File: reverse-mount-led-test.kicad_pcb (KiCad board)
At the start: 2 copper layers, 12.7 x 12.7 mm, 9 parts, among them J1 Conn_01x02

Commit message: setup design rules
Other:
- net class Default: clearance 0.2 -> 0.254; trace_width 0.25 -> 0.254; via_dia 0.8 -> 0.6858; via_drill 0.4 -> 0.3302
- rule pad_to_mask_clearance: 0.051 -> 0.0508
- rule solder_mask_min_width: 0.25 -> 0.254
- rule trace_clearance: 0.2 -> 0.254
- rule trace_min: 0.2 -> 0.1524
- rule via_min_drill: 0.3 -> 0.3302
- rule via_min_size: 0.4 -> 0.6858
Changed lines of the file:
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@@
   )
   (setup
-    (last_trace_width 0.25)
-    (trace_clearance 0.2)
+    (last_trace_width 0.254)
+    (trace_clearance 0.254)
     (zone_clearance 0.508)
     (zone_45_only no)
-    (trace_min 0.2)
+    (trace_min 0.1524)
     (segment_width 0.2)
     (edge_width 0.15)
-    (via_size 0.8)
-    (via_drill 0.4)
-    (via_min_size 0.4)
-    (via_min_drill 0.3)
+    (via_size 0.6858)
+    (via_drill 0.3302)
+    (via_min_size 0.6858)
+    (via_min_drill 0.3302)
     (uvia_size 0.3)
     (uvia_drill 0.1)
@@
     (pad_size 1.524 1.524)
     (pad_drill 0.762)
-    (pad_to_mask_clearance 0.051)
-    (solder_mask_min_width 0.25)
+    (pad_to_mask_clearance 0.0508)
+    (solder_mask_min_width 0.254)
     (aux_axis_origin 0 0)
     (visible_elements FFFFFF7F)
@@
   (net 6 "Net-(D4-Pad1)")
   (net_class Default "This is the default net class."
-    (clearance 0.2)
-    (trace_width 0.25)
-    (via_dia 0.8)
-    (via_drill 0.4)
+    (clearance 0.254)
+    (trace_width 0.254)
+    (via_dia 0.6858)
+    (via_drill 0.3302)
     (uvia_dia 0.3)
     (uvia_drill 0.1)

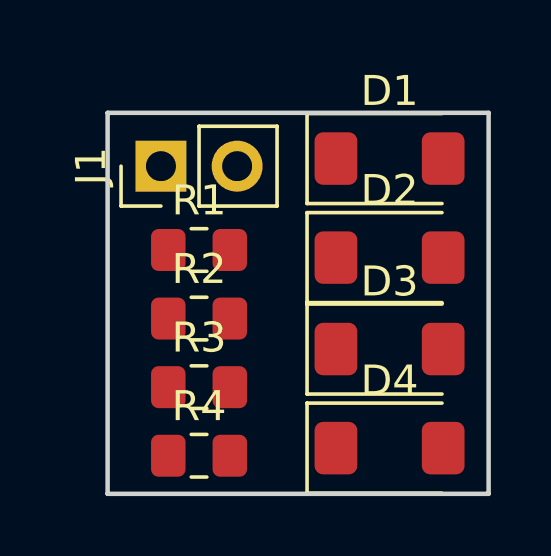
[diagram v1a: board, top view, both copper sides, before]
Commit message: layout done
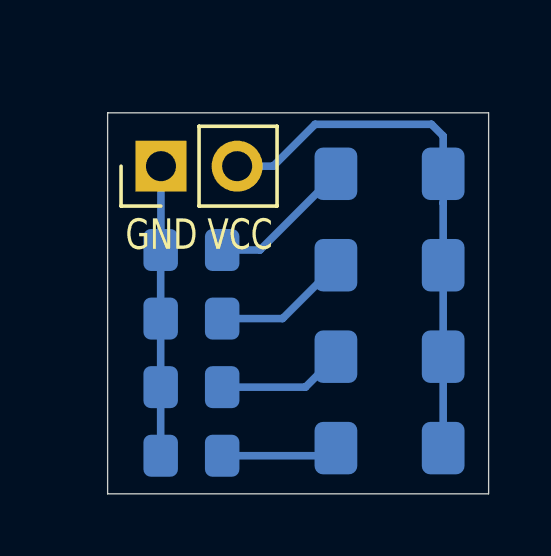
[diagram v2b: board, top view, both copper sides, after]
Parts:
- D1, D2, D3, D4, R1, R2, R3, R4: moved to B.Cu
- moved D1 0.51 mm to (161.8, 103.6)
- moved R1 0.25 mm to (155.2, 106.2)
- moved R2 0.25 mm to (155.2, 108.5)
- moved R3 0.25 mm to (155.2, 110.7)
- moved R4 0.25 mm to (155.2, 113.0)
- moved D2 0.25 mm to (161.8, 106.7)
- moved D3 0.25 mm to (161.8, 109.7)
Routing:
- net VCC: track 0.00 -> 18.0 mm
- net GND: track 0.00 -> 9.67 mm
- net Net-(D1-Pad1): track 0.00 -> 4.86 mm
- net Net-(D2-Pad1): track 0.00 -> 4.53 mm
- net Net-(D3-Pad1): track 0.00 -> 4.21 mm
- net Net-(D4-Pad1): track 0.00 -> 3.90 mm
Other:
- board text added: "GND VCC"
